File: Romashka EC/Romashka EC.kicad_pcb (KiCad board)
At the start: 2 copper layers, 228.6 x 76.2 mm, 128 parts, among them J1 USB_C_Receptacle_USB2.0_16P, J2 JSB USB, J3 SOICbite, SW1 EC_SW, SW10 EC_SW, SW11 EC_SW, SW12 EC_SW, SW13 EC_SW, SW14 EC_SW, SW15 EC_SW, SW16 EC_SW, SW17 EC_SW, SW18 EC_SW, SW19 EC_SW, SW2 EC_SW, SW20 EC_SW, SW21 EC_SW, SW22 EC_SW, SW23 EC_SW, SW24 EC_SW, SW25 EC_SW, SW26 EC_SW, SW27 EC_SW, SW28 EC_SW, SW29 EC_SW, SW3 EC_SW, SW30 EC_SW, SW31 EC_SW, SW32 EC_SW, SW35 EC_SW, SW36 EC_SW, SW38 EC_SW, SW39 EC_SW, SW4 EC_SW, SW40 EC_SW, SW42 EC_SW, SW43 EC_SW, SW44 EC_SW, SW45 EC_SW, SW47 EC_SW, SW49 EC_SW, SW5 EC_SW, SW6 EC_SW, SW7 EC_SW, SW8 EC_SW, SW9 EC_SW, U1 STM32G474CBTx, U2 USBLC6-2P6, U3 TPS7A2033, U4 OPA2365, U5 4052, U6 OPA2365, U7 4052, Y1 8Mhz 12pF

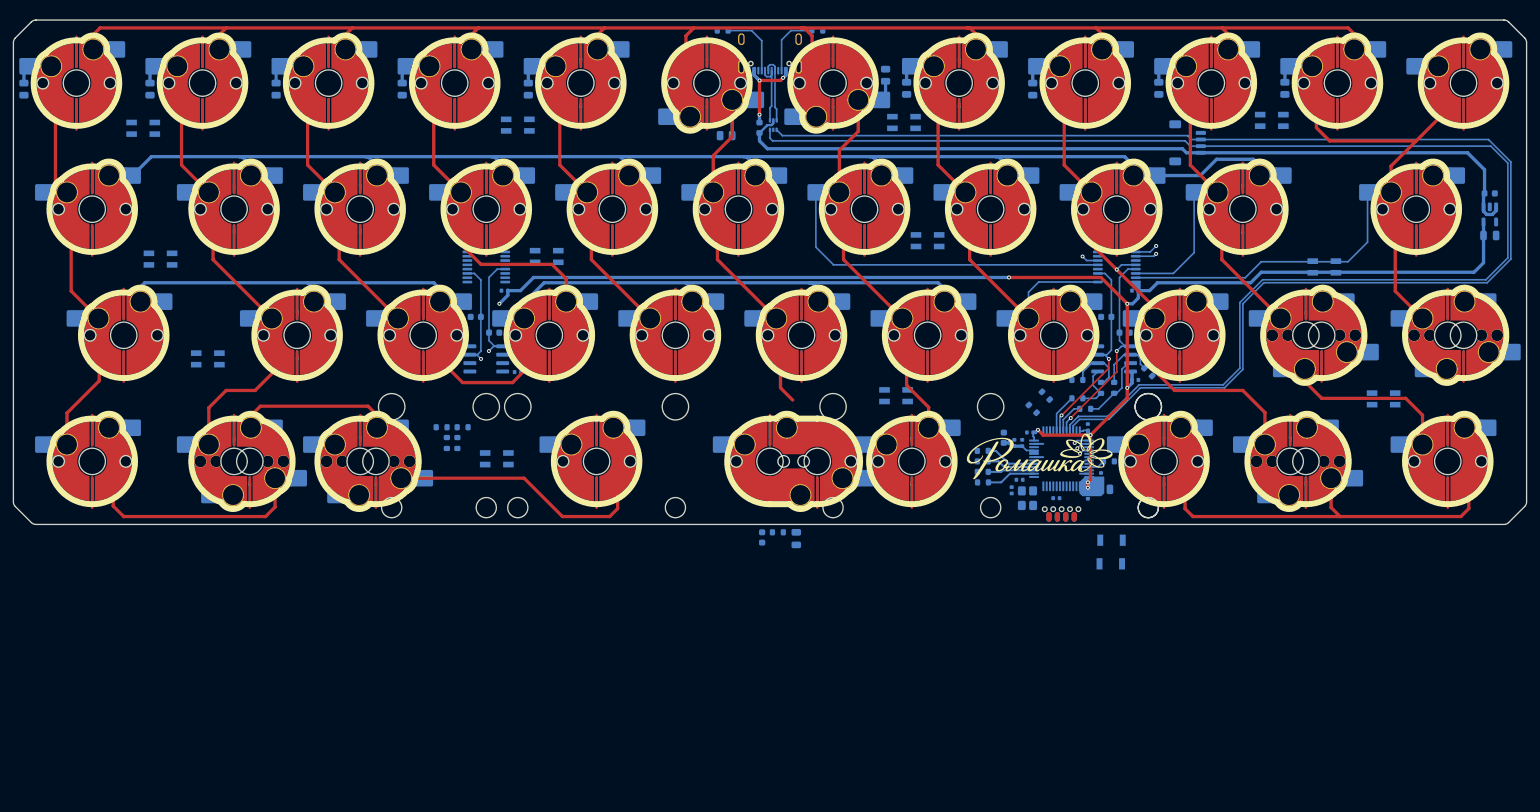
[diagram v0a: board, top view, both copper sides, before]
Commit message: 20.04.2026: setup
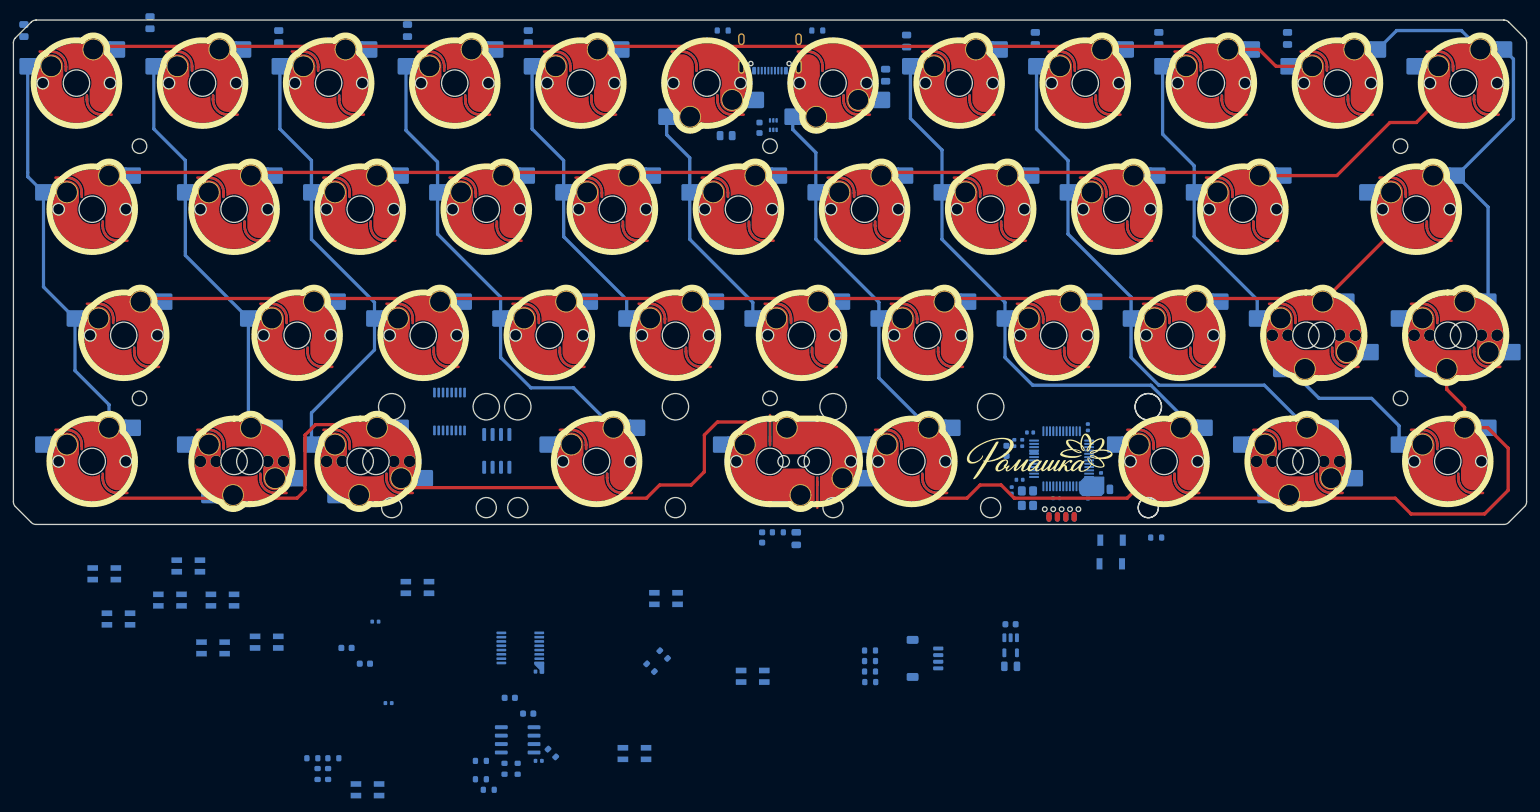
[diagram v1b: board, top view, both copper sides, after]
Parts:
- added REF**: m2 hole, Kicad footprints:m2 hole, F.Cu at (127.0, 31.8)
- added REF**: m2 hole, Kicad footprints:m2 hole, F.Cu at (222.2, 31.8)
- added REF**: m2 hole, Kicad footprints:m2 hole, F.Cu at (31.8, 31.8)
- added REF**: m2 hole, Kicad footprints:m2 hole, F.Cu at (222.2, 69.8)
- added REF**: m2 hole, Kicad footprints:m2 hole, F.Cu at (31.8, 69.8)
- added REF**: m2 hole, Kicad footprints:m2 hole, F.Cu at (127.0, 69.8)
- SW1, SW10, SW13, SW14, SW15, SW16, SW17, SW18, SW19, SW2, SW20, SW21, SW22, SW24, SW25, SW26, SW28, SW29, SW3, SW30, SW31, SW32, SW4, SW42, SW5, SW8, SW9: footprint Kicad footprints:ecs_pad_1U_hybrid_hotswap_V2 -> Kicad footprints:ecs_pad_1U_hybrid_hotswap_V3
- SW11, SW12, SW23, SW35, SW38, SW40, SW6, SW7: footprint Kicad footprints:ecs_pad_1U_hybrid_hotswap_V2 -> Kicad footprints:ecs_pad_1U_hybrid_hotswap_V3_switched_sides
- SW27: footprint Kicad footprints:ecs_pad_1U_hybrid_hotswap_V2_switched_sides -> Kicad footprints:ecs_pad_1U_hybrid_hotswap_V3
- SW36, SW43, SW44, SW45, SW47: footprint Kicad footprints:ecs_pad_hybrid_hotswap_2.381_V2 -> Kicad footprints:ecs_pad_hybrid_hotswap_2.381_V3
- SW39: footprint Kicad footprints:ecs_pad_1U_hybrid_hotswap_V2_switched_sides -> Kicad footprints:ecs_pad_1U_hybrid_hotswap_V3_switched_sides
- moved D9 174.3 mm to (44.3, 100.3)
- moved D8 169.5 mm to (51.0, 106.7)
- moved D10 131.1 mm to (42.9, 107.6)
- moved C27 106.9 mm to (87.7, 115.1)
- moved C24 106.9 mm to (92.1, 111.1)
- moved C25 106.9 mm to (90.5, 117.5)
- moved C26 106.9 mm to (92.1, 124.6)
- moved R23 106.9 mm to (86.9, 125.8)
- moved R24 106.9 mm to (83.3, 124.6)
- moved R28 106.9 mm to (88.9, 125.8)
- moved R29 106.9 mm to (94.0, 123.4)
- moved R5 106.9 mm to (83.3, 127.4)
- moved R6 106.9 mm to (84.5, 129.0)
- moved U6 106.9 mm to (88.9, 121.4)
- moved U7 106.9 mm to (89.3, 107.6)
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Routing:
- net D-: track 212.1 -> 0.00 mm
- net D+: track 210.8 -> 0.00 mm
- net +3.3V: track 207.4 -> 0.00 mm, vias 8 -> 0
- net +5V: track 124.9 -> 0.00 mm
- net ROW3: track 168.0 -> 224.9 mm
- net ROW0: track 240.0 -> 185.2 mm
- net COL6: track 105.7 -> 55.5 mm
- net COL10: track 108.0 -> 62.1 mm
- net ROW2: track 153.6 -> 197.1 mm
- net DISCHARGE3: track 32.5 -> 0.00 mm, vias 2 -> 0
- net DISCHARGE2: track 30.9 -> 0.00 mm, vias 2 -> 0
- net COL7: track 56.1 -> 82.0 mm
- net COL2: track 41.2 -> 67.0 mm
- net COL3: track 47.6 -> 71.4 mm
- net COL9: track 86.5 -> 66.0 mm
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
